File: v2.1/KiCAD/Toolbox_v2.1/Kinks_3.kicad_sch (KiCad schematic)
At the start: 31 parts, among them J30 Kinks_OUT_Noise, J31 Kinks_OUT_S&H, J32 Kinks_S&H_IN, J33 Kinks_S&H_TRIG, Q1 MMBT3904, Q2 MMBT3904, Q3 MMBFJ310, U11 TL074, U7 TL074

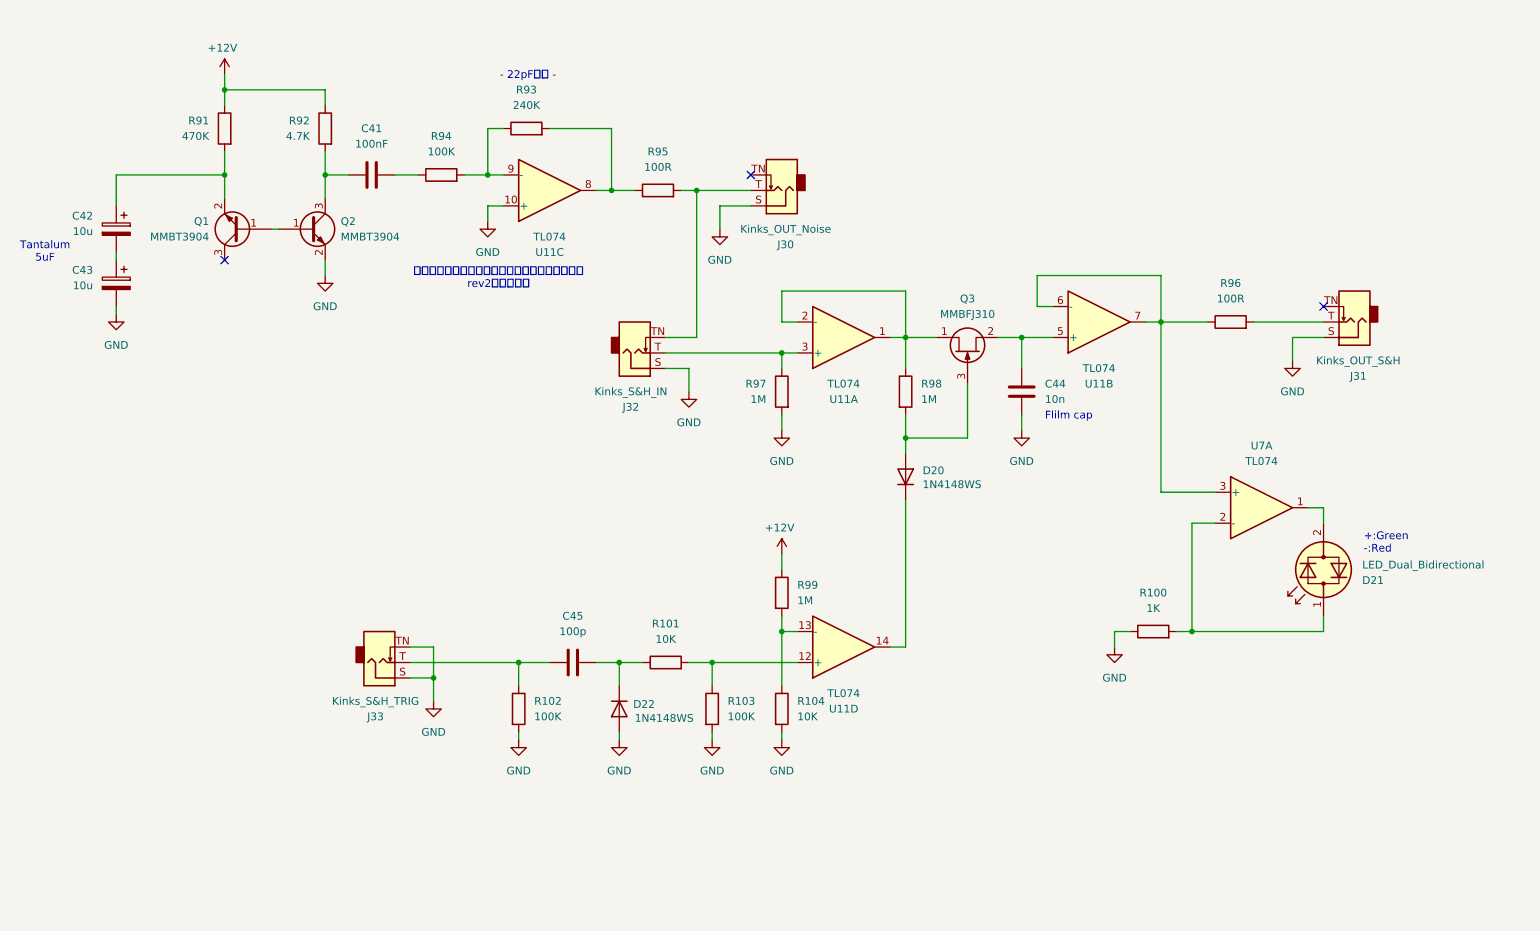
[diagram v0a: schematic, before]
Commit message: v2.1 Update
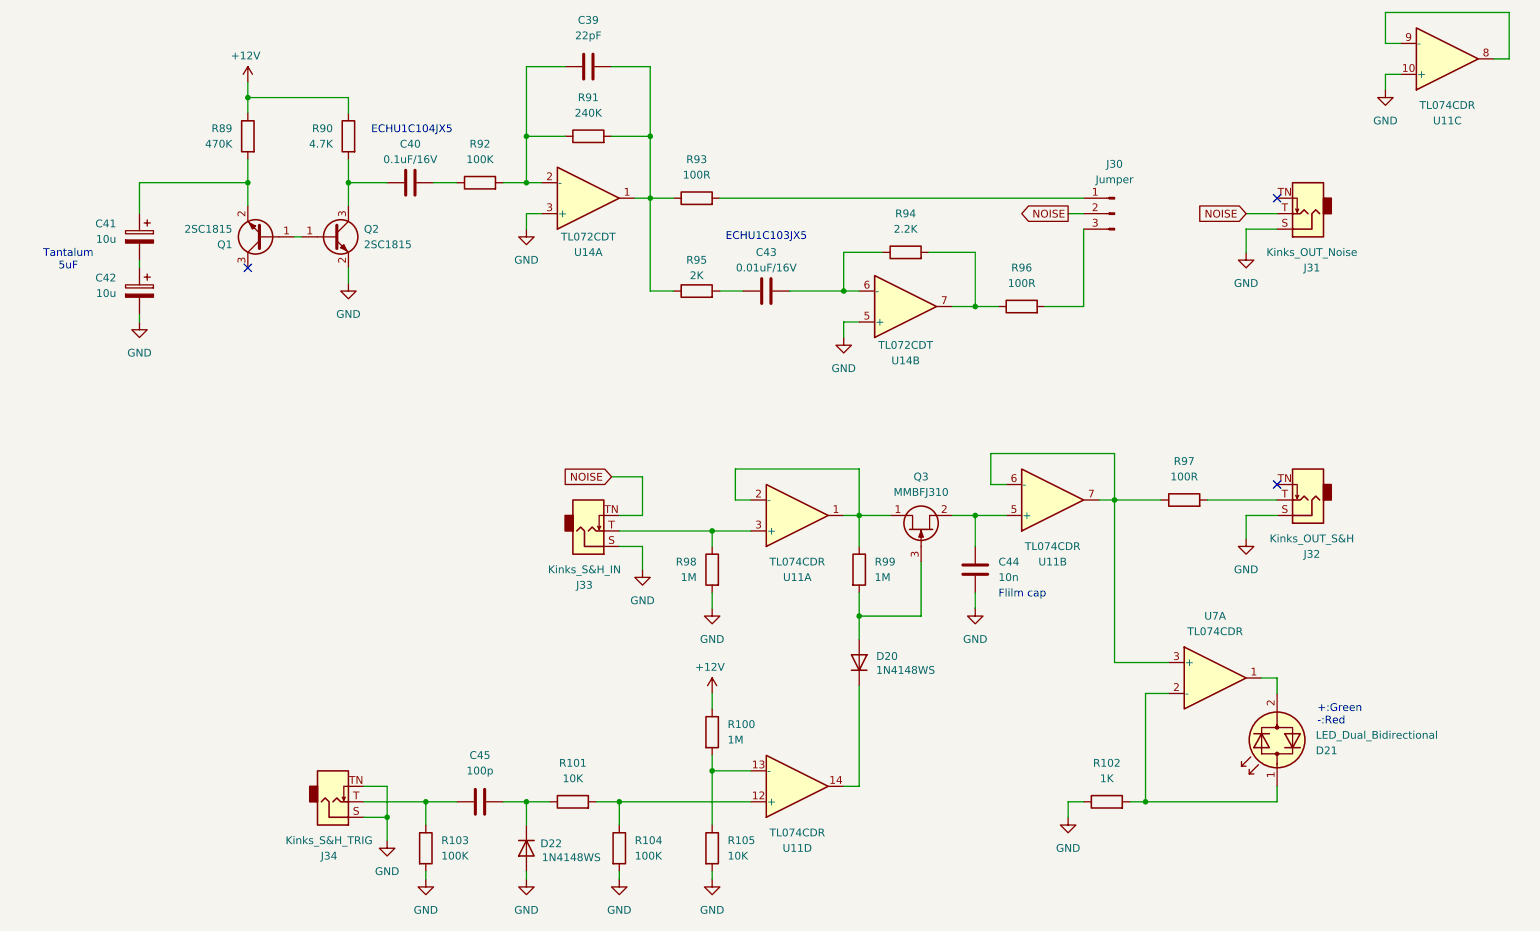
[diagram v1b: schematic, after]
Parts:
- added C39: 22pF, Capacitor_SMD:C_0603_1608Metric, symbol Device:C
- added C43: 0.01uF/16V, Capacitor_SMD:C_0805_2012Metric_Pad1.18x1.45mm_HandSolder, symbol Device:C
- added J30: Jumper, Connector_PinHeader_2.54mm:PinHeader_1x03_P2.54mm_Vertical, symbol Connector:Conn_01x03_Pin
- added R94: 2.2K, Resistor_SMD:R_0603_1608Metric, symbol Device:R
- added R95: 2K, Resistor_SMD:R_0603_1608Metric, symbol Device:R
- added R96: 100R, Resistor_SMD:R_0402_1005Metric, symbol Device:R
- added U14: TL072CDT, Package_SO:SOIC-8_3.9x4.9mm_P1.27mm, symbol Amplifier_Operational:TL072
- C40: renamed from C41; value 100nF -> 0.1uF/16V; footprint Capacitor_THT:C_Rect_L7.2mm_W2.5mm_P5.00mm_FKS2_FKP2_MKS2_MKP2 -> Capacitor_SMD:C_1210_3225Metric_Pad1.33x2.70mm_HandSolder
- Q1, Q2: value MMBT3904 -> 2SC1815; LCSC C20526 -> C20069143
- Q3: LCSC (none) -> C33416
- U11, U7: value TL074 -> TL074CDR; footprint Package_SO:TSSOP-14_4.4x5mm_P0.65mm -> Package_SO:SOIC-14_3.9x8.7mm_P1.27mm; LCSC C4370424 -> C12594
- renumbered C42 to C41, C43 to C42, J30 to J31, J31 to J32, J32 to J33, J33 to J34, R99 to R100, R100 to R102, R102 to R103, R103 to R104, R104 to R105, R91 to R89, R92 to R90, R93 to R91, R94 to R92, R95 to R93, R96 to R97, R97 to R98, R98 to R99
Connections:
- net GND: now also U14.3 (+), U14.5 (+)
- net at R91.2, R93.1: now also C39.2, R95.1, U14.1; no longer U11.8
- net NOISE: now reaches J31.T, J33.TN
- net NOISE: now also J30.2 (Pin_2); no longer R93.2
- net at R91.1, R92.2: now also C39.1, U14.2 (-); no longer U11.9 (-)
- new net: R94.2, R96.1, U14.7
- new net: J30.3 (Pin_3), R96.2
- new net: C43.1, R95.2
- new net: J30.1 (Pin_1), R93.2
- new net: U11.8, U11.9 (-)
- new net: C43.2, R94.1, U14.6 (-)
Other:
- note added: "ECHU1C103JX5"
- note added: "ECHU1C104JX5"
- note removed: "- 22pF並列 -"
- note removed: "ノイズ周りだけオペアンプ分けたほうがいいかも rev2で対応予定"
- moved on the sheet: C40, C41, C42, C44, C45, D20, D21, D22, J31, J32, J33, J34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
